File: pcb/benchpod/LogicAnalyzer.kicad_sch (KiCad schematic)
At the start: 50 parts, among them U18 SN74LVC2G66DCTR, U19 SN74LVC2G66DCTR, U20 SN74LVC2G66DCTR, U21 SN74LVC2G66DCTR, U22 SRV05-4.TCT, U23 SRV05-4.TCT, U24 PCA9555PW,118, U25 SRV05-4.TCT

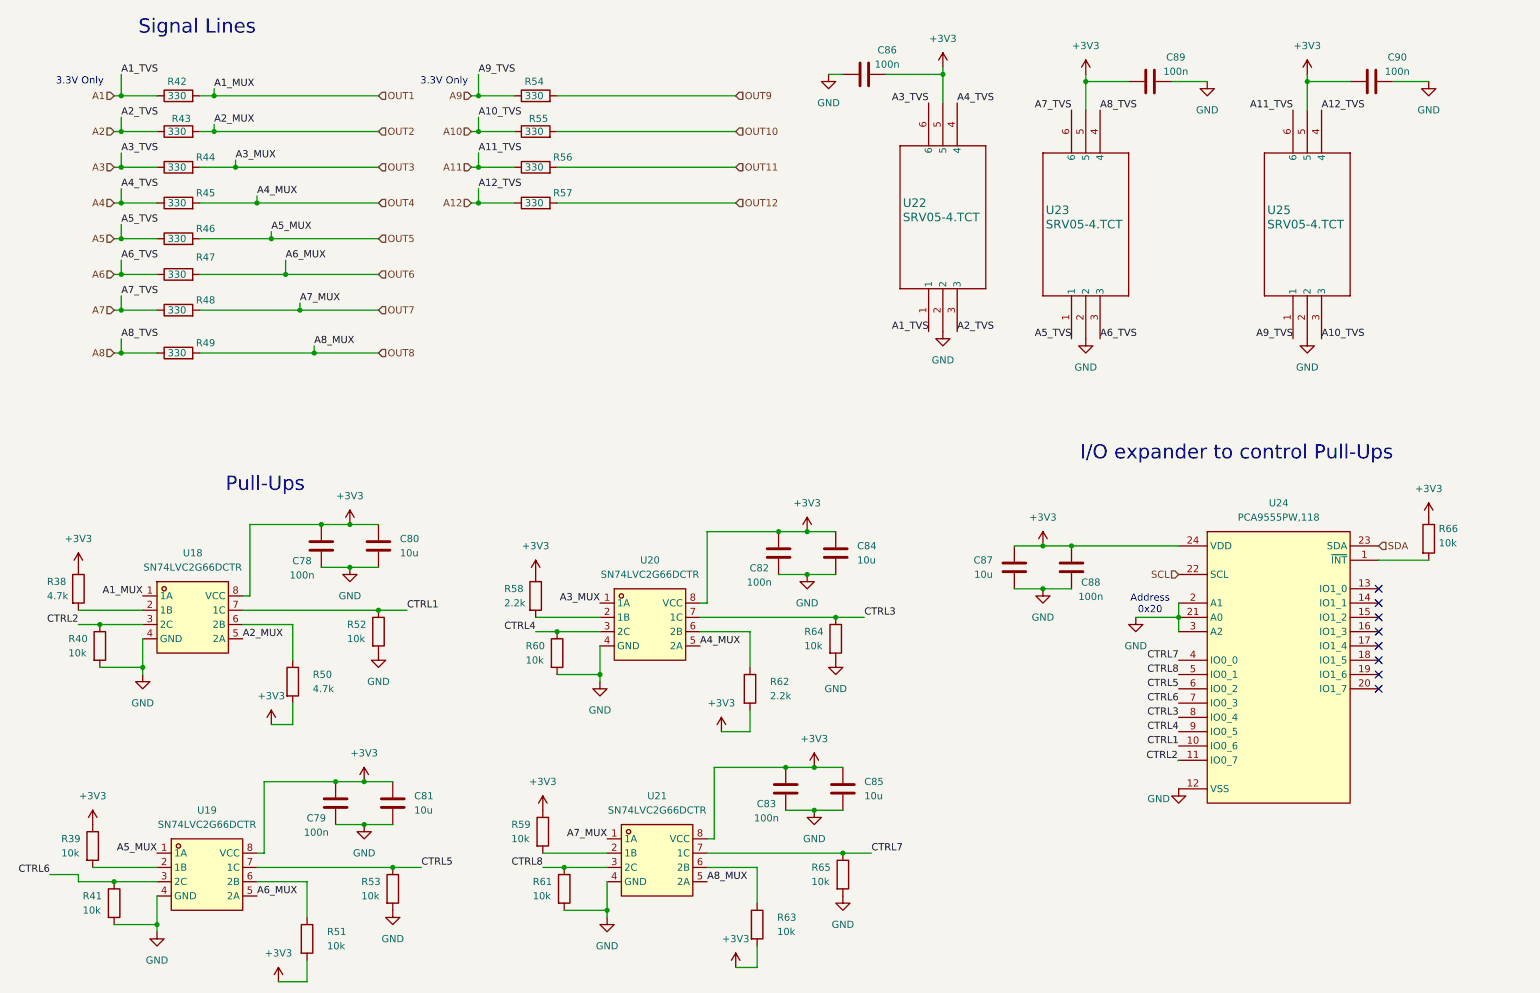
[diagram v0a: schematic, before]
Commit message: v2.0.0
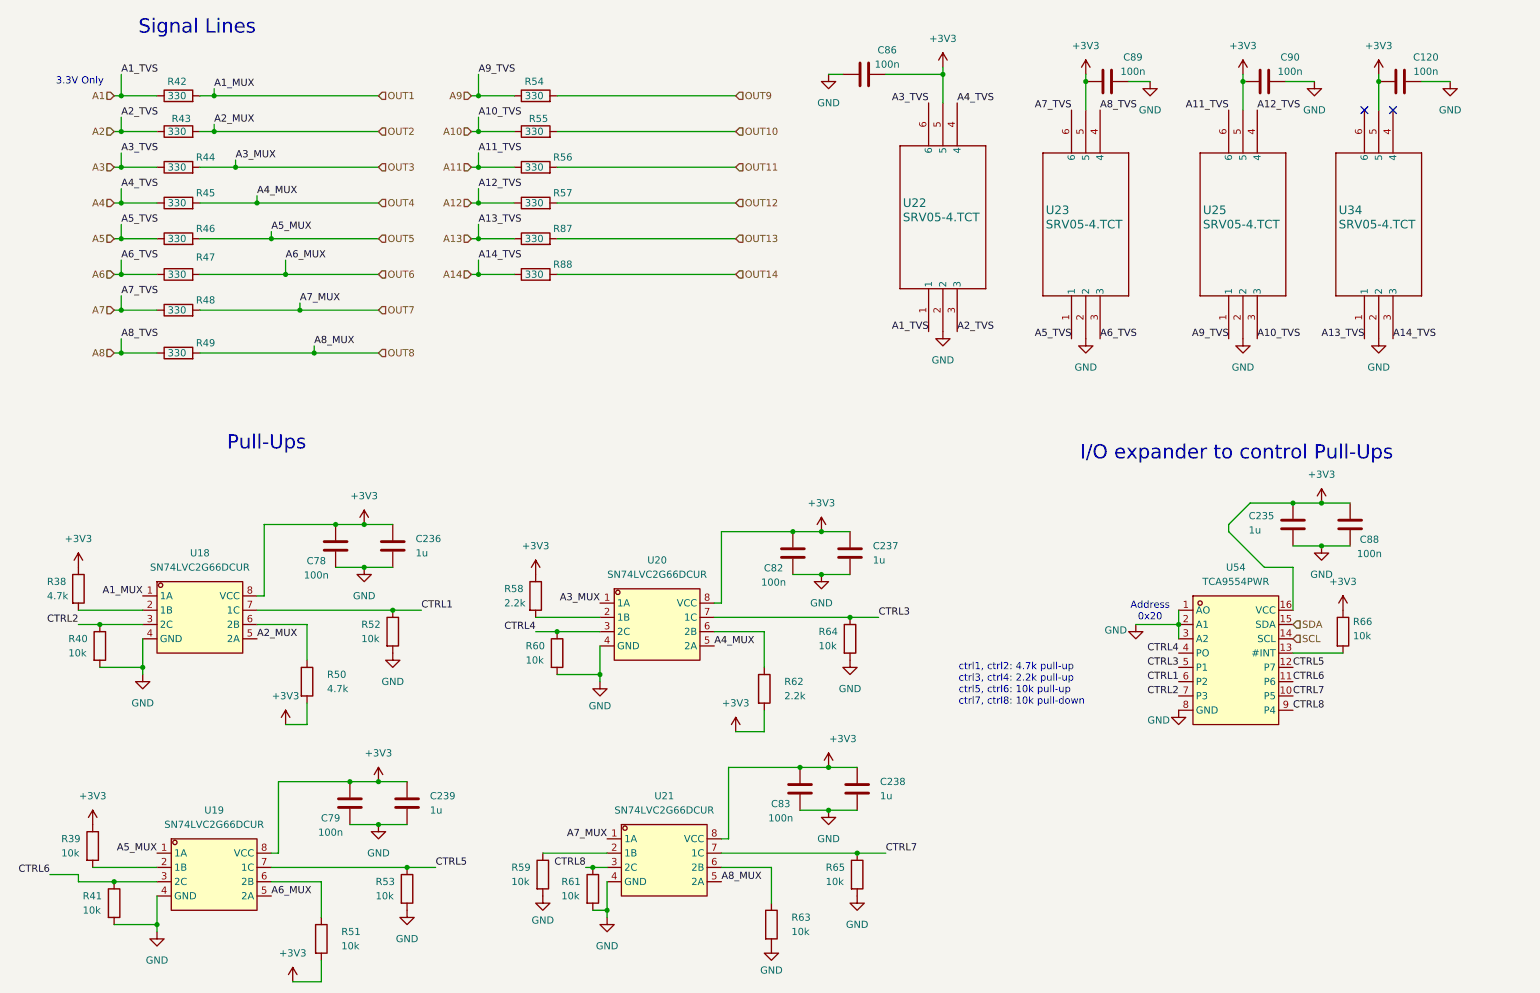
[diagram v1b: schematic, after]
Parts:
- removed C80, C81, C84, C85, C87: 10u, Capacitor_SMD:C_0603_1608Metric, symbol Device:C
- removed U18, U19, U20, U21: SN74LVC2G66DCTR, lcsc:SM-8_L3.0-W2.8-P0.65-LS4.0-BR, symbol lcsc_lib:SN74LVC2G66DCTR
- removed U24: PCA9555PW,118, lcsc:TSSOP-24_L7.8-W4.4-P0.65-LS6.4-BL, symbol lcsc_lib:PCA9555PW,118
- added C120: 100n, Capacitor_SMD:C_0402_1005Metric, symbol Device:C
- added C235, C236, C237, C238, C239: 1u, Capacitor_SMD:C_0402_1005Metric, symbol Device:C
- added R87, R88: 330, Resistor_SMD:R_0402_1005Metric, symbol Device:R
- added U18, U19, U20, U21: SN74LVC2G66DCUR, lcsc:VSSOP-8_L2.1-W2.4-P0.50-LS3.2-BR, symbol lcsc_lib:SN74LVC2G66DCUR
- added U34: SRV05-4.TCT, lcsc:SOT-23-6_L2.9-W1.6-P0.95-LS2.8-BR, symbol edward_lib:SRV05-4.TCT
- added U54: TCA9554PWR, lcsc:TSSOP-16_L5.0-W4.4-P0.65-LS6.4-TL, symbol lcsc_lib:TCA9554PWR
- C78, C79, C82, C83, C86, C88, C89, C90: footprint Capacitor_SMD:C_0603_1608Metric -> Capacitor_SMD:C_0402_1005Metric; LCSC C14663 -> C307331
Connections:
- net +3V3: now also C120.1, C235.2, C236.2, C237.2, C238.2, C239.2, U18.8 (VCC), U19.8 (VCC), U20.8 (VCC), U21.8 (VCC), U34.5, U54.16 (VCC); no longer R59.1, R63.2
- net CTRL1: now also U18.7 (1C), U54.6 (P2)
- net CTRL2: now also U18.3 (2C), U54.7 (P3)
- net CTRL3: now also U20.7 (1C), U54.5 (P1)
- net CTRL4: now also U20.3 (2C), U54.4 (PO)
- net CTRL5: now also U19.7 (1C), U54.12 (P7)
- net CTRL6: now also U19.3 (2C), U54.11 (P6)
- net CTRL7: now also U21.7 (1C), U54.10 (P5)
- net CTRL8: now also U21.3 (2C), U54.9 (P4)
- net GND: now also R59.2, R63.2, C120.2, C235.1, C236.1, C237.1, C238.1, C239.1, U18.4 (GND), U19.4 (GND), U20.4 (GND), U21.4 (GND), U34.2, U54.1 (AO), U54.2 (A1), U54.3 (A2), U54.8 (GND)
- net OUT1: now also U18.1 (1A)
- net OUT2: now also U18.5 (2A)
- net OUT3: now also U20.1 (1A)
- net OUT4: now also U20.5 (2A)
- net OUT5: now also U19.1 (1A)
- net OUT6: now also U19.5 (2A)
- net OUT7: now also U21.1 (1A)
- net OUT8: now also U21.5 (2A)
- net SCL: now also U54.14 (SCL)
- net SDA: now also U54.15 (SDA)
- net at R58.2: now also U20.2 (1B)
- net at R38.2: now also U18.2 (1B)
- net at R62.1: now also U20.6 (2B)
- net at R66.2: now also U54.13 (#INT)
- net at R50.1: now also U18.6 (2B)
- net at R63.1: now also U21.6 (2B)
- net at R39.2: now also U19.2 (1B)
- net at R51.1: now also U19.6 (2B)
- new net: R59.1, U21.2 (1B)
- new net A13: R87.1, U34.1
- new net A14: R88.1, U34.3
- new net OUT13: R87.2
- new net OUT14: R88.2
- no-connect marks 8 -> 2
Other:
- note added: "ctrl1, ctrl2: 4.7k pull-up ctrl3, ctrl4: 2.2k pull-up ctrl5, ctrl6: 10k pull-up ctrl7, ctrl8: 10k pull-down"
- moved on the sheet: C78, C79, C82, C83, C88, C89, C90, R50, R51, R52, R53, R59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
